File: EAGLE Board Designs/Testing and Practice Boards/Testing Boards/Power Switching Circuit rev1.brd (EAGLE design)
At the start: 93.4 x 66.3 mm, 50 parts, among them K1 J115F11A6*, Q1 SIR638ADP, Q2 SIR638ADP, Q3 SIR638ADP, Q4 SIR638ADP, U1 LTC4421, X1 CONNECTOR-3, X100 CONNECTOR-4AUTOSPORT, X101 CONNECTOR-4AUTOSPORT

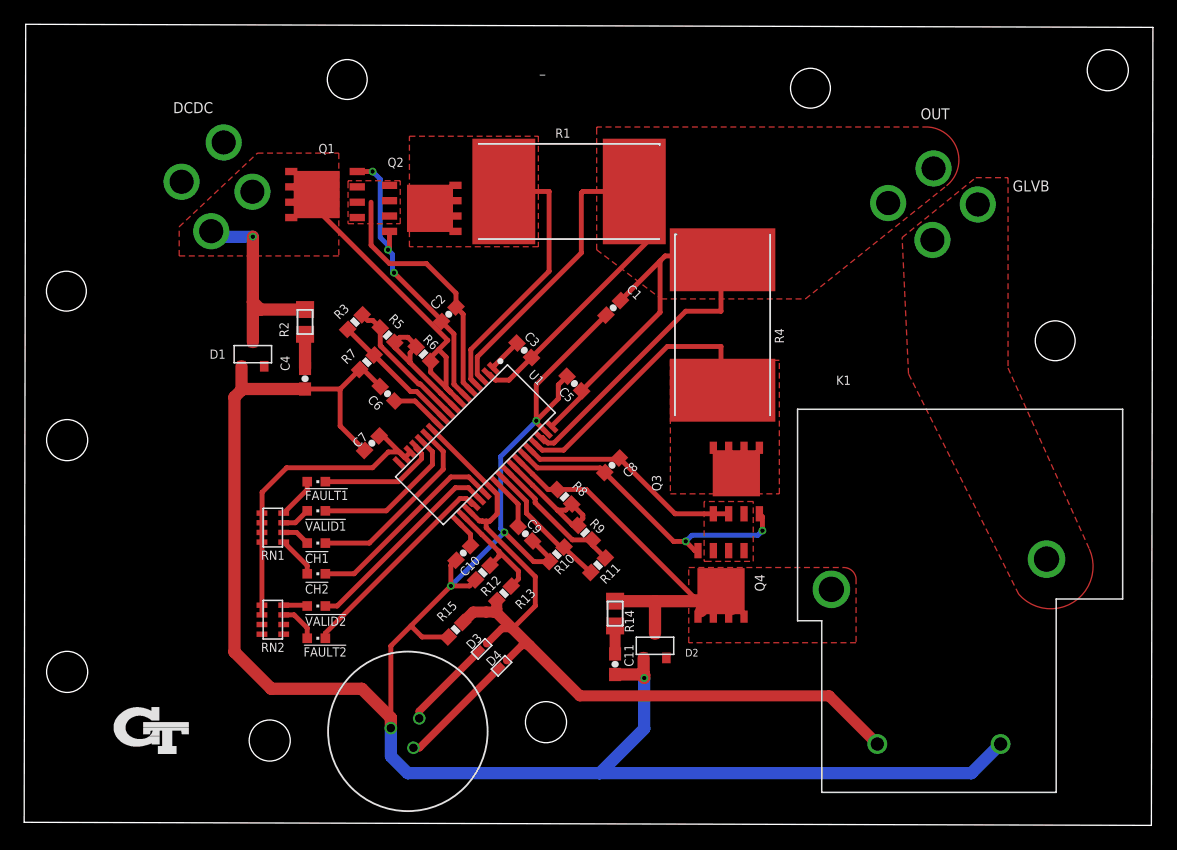
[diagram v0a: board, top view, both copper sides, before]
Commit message: Minor fixes
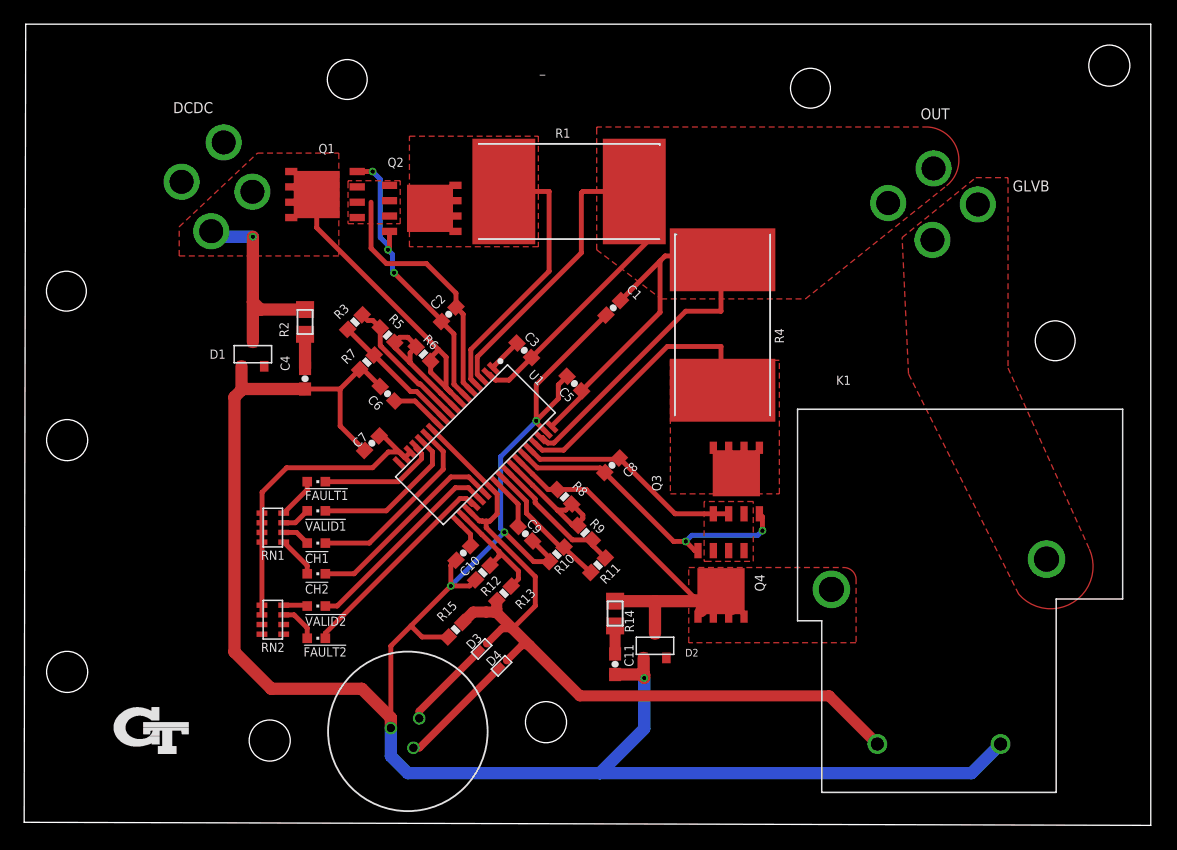
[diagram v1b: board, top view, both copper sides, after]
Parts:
- moved U$4 0.40 mm to (61.7, 36.1)
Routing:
- net DCDC: track 44.3 -> 43.7 mm
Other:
- board size 93.4 x 66.3 mm -> 93.2 x 66.3 mm
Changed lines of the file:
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@@
 <drawing>
 <settings>
-<setting alwaysvectorfont="yes"/>
+<setting alwaysvectorfont="no"/>
 <setting verticaltext="up"/>
 </settings>
@@
 <layer number="17" name="Pads" color="2" fill="1" visible="yes" active="yes"/>
 <layer number="18" name="Vias" color="2" fill="1" visible="yes" active="yes"/>
-<layer number="19" name="Unrouted" color="6" fill="1" visible="no" active="yes"/>
+<layer number="19" name="Unrouted" color="6" fill="1" visible="yes" active="yes"/>
 <layer number="20" name="Dimension" color="24" fill="1" visible="yes" active="yes"/>
 <layer number="21" name="tPlace" color="7" fill="1" visible="yes" active="yes"/>
@@
 <layer number="26" name="bNames" color="7" fill="1" visible="yes" active="yes"/>
 <layer number="27" name="tValues" color="7" fill="1" visible="yes" active="yes"/>
-<layer number="28" name="bValues" color="7" fill="1" visible="no" active="yes"/>
-<layer number="29" name="tStop" color="7" fill="3" visible="yes" active="yes"/>
-<layer number="30" name="bStop" color="7" fill="6" visible="yes" active="yes"/>
-<layer number="31" name="tCream" color="7" fill="4" visible="yes" active="yes"/>
+<layer number="28" name="bValues" color="7" fill="1" visible="yes" active="yes"/>
+<layer number="29" name="tStop" color="7" fill="3" visible="no" active="yes"/>
+<layer number="30" name="bStop" color="7" fill="6" visible="no" active="yes"/>
+<layer number="31" name="tCream" color="7" fill="4" visible="no" active="yes"/>
 <layer number="32" name="bCream" color="7" fill="5" visible="no" active="yes"/>
 <layer number="33" name="tFinish" color="6" fill="3" visible="no" active="yes"/>
 <layer number="34" name="bFinish" color="6" fill="6" visible="no" active="yes"/>
-<layer number="35" name="tGlue" color="7" fill="4" visible="yes" active="yes"/>
+<layer number="35" name="tGlue" color="7" fill="4" visible="no" active="yes"/>
 <layer number="36" name="bGlue" color="7" fill="5" visible="no" active="yes"/>
 <layer number="37" name="tTest" color="7" fill="1" visible="no" active="yes"/>
@@
 <layer number="39" name="tKeepout" color="4" fill="11" visible="yes" active="yes"/>
 <layer number="40" name="bKeepout" color="1" fill="11" visible="yes" active="yes"/>
-<layer number="41" name="tRestrict" color="4" fill="10" visible="yes" active="yes"/>
-<layer number="42" name="bRestrict" color="1" fill="10" visible="yes" active="yes"/>
+<layer number="41" name="tRestrict" color="4" fill="10" visible="no" active="yes"/>
+<layer number="42" name="bRestrict" color="1" fill="10" visible="no" active="yes"/>
 <layer number="43" name="vRestrict" color="2" fill="10" visible="no" active="yes"/>
-<layer number="44" name="Drills" color="7" fill="1" visible="yes" active="yes"/>
-<layer number="45" name="Holes" color="7" fill="1" visible="yes" active="yes"/>
+<layer number="44" name="Drills" color="7" fill="1" visible="no" active="yes"/>
+<layer number="45" name="Holes" color="7" fill="1" visible="no" active="yes"/>
 <layer number="46" name="Milling" color="3" fill="1" visible="no" active="yes"/>
 <layer number="47" name="Measures" color="7" fill="1" visible="no" active="yes"/>
@@
 <layer number="50" name="dxf" color="7" fill="1" visible="no" active="no"/>
 <layer number="51" name="tDocu" color="7" fill="1" visible="yes" active="yes"/>
-<layer number="52" name="bDocu" color="7" fill="1" visible="no" active="yes"/>
+<layer number="52" name="bDocu" color="7" fill="1" visible="yes" active="yes"/>
 <layer number="53" name="tGND_GNDA" color="7" fill="9" visible="no" active="no"/>
 <layer number="54" name="bGND_GNDA" color="1" fill="9" visible="no" active="no"/>
@@
 <board>
 <plain>
-<wire x1="-28.067" y1="-26.543" x2="65.202" y2="-26.797" width="0" layer="20"/>
-<wire x1="65.202" y1="-26.797" x2="65.329" y2="39.233" width="0" layer="20"/>
-<wire x1="65.329" y1="39.233" x2="-27.94" y2="39.487" width="0" layer="20"/>
-<wire x1="-27.94" y1="39.487" x2="-28.067" y2="-26.543" width="0" layer="20"/>
+<wire x1="-28.067" y1="-26.543" x2="65.151" y2="-26.797" width="0" layer="20"/>
+<wire x1="65.151" y1="-26.797" x2="65.151" y2="39.497" width="0" layer="20"/>
+<wire x1="65.151" y1="39.497" x2="-27.94" y2="39.497" width="0" layer="20"/>
+<wire x1="-27.94" y1="39.497" x2="-28.067" y2="-26.543" width="0" layer="20"/>
 <text x="-4.953" y="-12.827" size="0.762" layer="21" font="vector">!FAULT2</text>
 <text x="-4.826" y="0.127" size="0.762" layer="21" font="vector">!FAULT1</text>
@@
 <element name="U$1" library="HyTechDevices" package="MOUNTING_M3" value="" x="-24.511" y="-14.097" smashed="yes"/>
 <element name="U$3" library="HyTechDevices" package="MOUNTING_M3" value="" x="-24.511" y="5.08" smashed="yes"/>
-<element name="U$4" library="HyTechDevices" package="MOUNTING_M3" value="" x="61.595" y="35.687" smashed="yes"/>
+<element name="U$4" library="HyTechDevices" package="MOUNTING_M3" value="" x="61.722" y="36.068" smashed="yes"/>
 </elements>
 <signals>
@@
 <wire x1="5.56790625" y1="11.595146875" x2="5.56790625" y2="11.91790625" width="0.4064" layer="1"/>
 <wire x1="5.56790625" y1="11.91790625" x2="6.223" y2="12.573" width="0.4064" layer="1"/>
-<wire x1="6.223" y1="12.573" x2="6.985" y2="13.335" width="0.4064" layer="1"/>
-<wire x1="-3.8608" y1="25.4" x2="-3.8608" y2="24.1808" width="0.4064" layer="1"/>
-<wire x1="-3.8608" y1="24.1808" x2="6.985" y2="13.335" width="0.4064" layer="1"/>
+<wire x1="-3.8608" y1="25.4" x2="-3.8608" y2="22.6568" width="0.4064" layer="1"/>
+<wire x1="-3.8608" y1="22.6568" x2="6.223" y2="12.573" width="0.4064" layer="1"/>
 <wire x1="-9.144" y1="16.51" x2="-9.144" y2="13.1953" width="1.016" layer="1"/>
 <via x="-9.144" y="21.908628125" extent="1-16" drill="0.35"/>
@@
 <vertex x="-1.27" y="22.987"/>
 <vertex x="3.048" y="22.987"/>
-<vertex x="3.048" y="22.987"/>
 <vertex x="3.048" y="26.543"/>
 <vertex x="-1.27" y="26.543"/>
@@
 <wire x1="7.6626375" y1="16.09439375" x2="7.6626375" y2="17.23739375" width="0.4064" layer="1"/>
 <wire x1="7.6626375" y1="17.23739375" x2="5.21503125" y2="19.685" width="0.4064" layer="1"/>
-<wire x1="5.21503125" y1="19.685" x2="2.159" y2="19.685" width="0.4064" layer="1"/>
-<wire x1="2.159" y1="19.685" x2="0.635" y2="21.209" width="0.4064" layer="1"/>
-<wire x1="0.635" y1="21.209" x2="0.635" y2="24.765" width="0.4064" layer="1"/>
+<wire x1="5.21503125" y1="19.685" x2="1.905" y2="19.685" width="0.4064" layer="1"/>
+<wire x1="1.905" y1="19.685" x2="0.635" y2="20.955" width="0.4064" layer="1"/>
+<wire x1="0.635" y1="20.955" x2="0.635" y2="24.765" width="0.4064" layer="1"/>
 </signal>
 <signal name="!SHDN">
